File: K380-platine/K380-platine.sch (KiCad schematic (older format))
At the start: 32 parts, among them J1 JST-PH 2, J2 Conn_01x23, J3 MicroMod-M.2E, J4 USB_C_Receptacle_USB2.0, J5 Conn_ARM_JTAG_SWD_10, Q1 PMost Enc FET -20V, Q2 Q_NMOS_DGS, SW1 EG1215AA, SW2 SW_Push, SW3 SW_Push, U1 XC6220B331MR, U2 MCP73831-2-OT

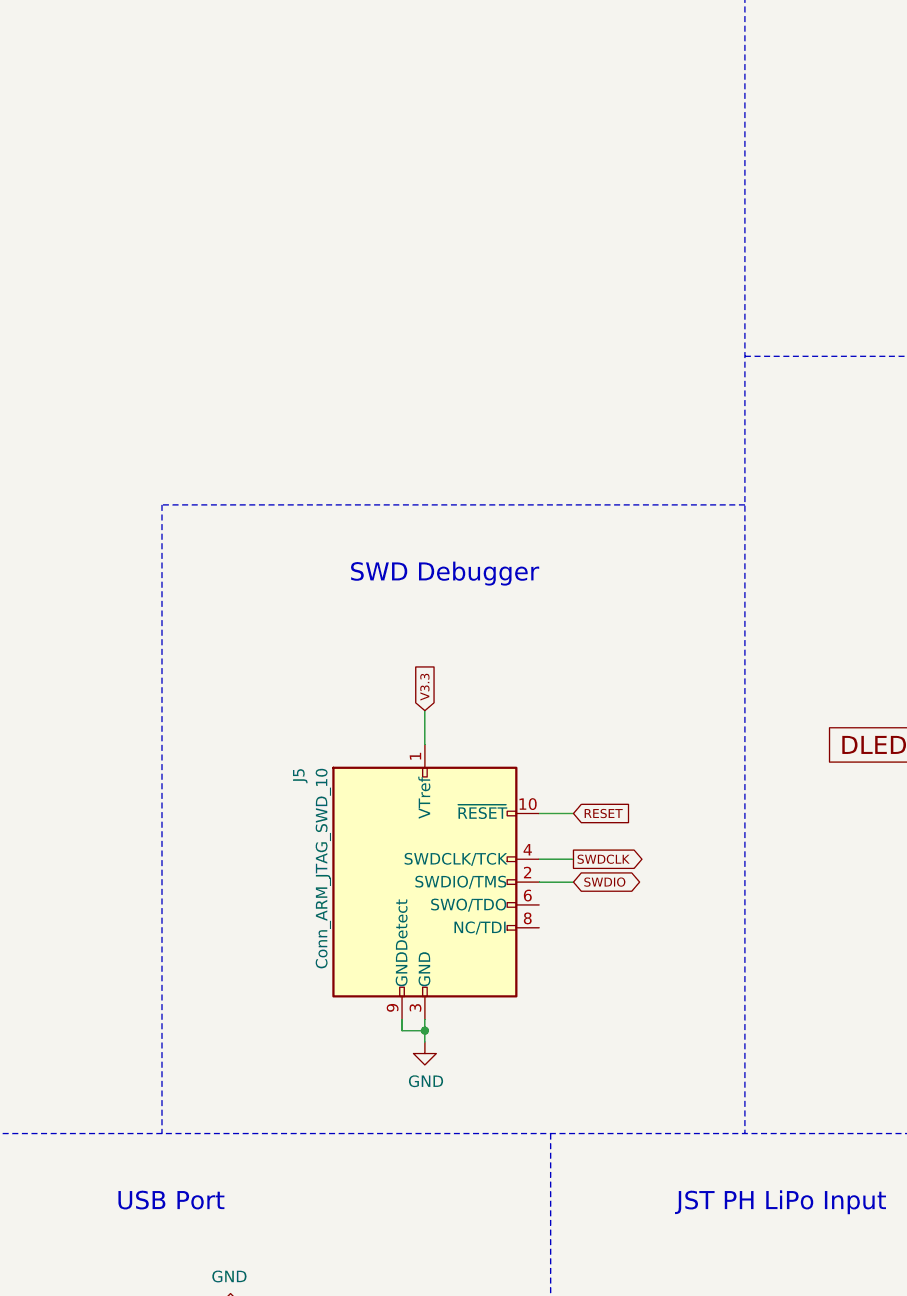
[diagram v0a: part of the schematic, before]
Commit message: Add test probes
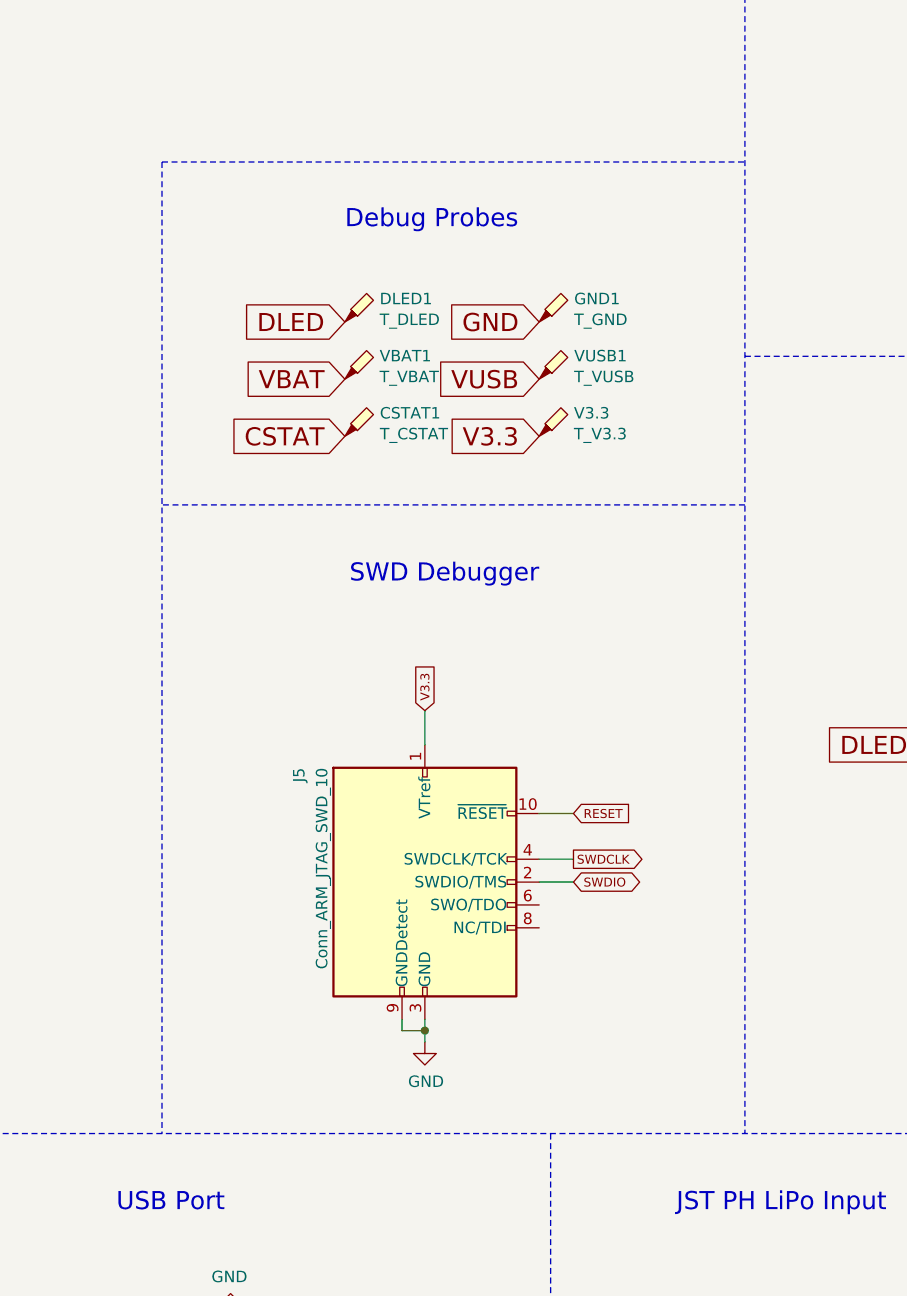
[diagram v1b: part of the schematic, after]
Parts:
- added CSTAT1: T_CSTAT, TestPoint:TestPoint_Pad_D1.0mm, symbol Connector:TestPoint_Probe
- added DLED1: T_DLED, TestPoint:TestPoint_Pad_D1.0mm, symbol Connector:TestPoint_Probe
- added GND1: T_GND, TestPoint:TestPoint_Pad_D1.0mm, symbol Connector:TestPoint_Probe
- added V3.3: T_V3.3, TestPoint:TestPoint_Pad_D1.0mm, symbol Connector:TestPoint_Probe
- added VBAT1: T_VBAT, TestPoint:TestPoint_Pad_D1.0mm, symbol Connector:TestPoint_Probe
- added VUSB1: T_VUSB, TestPoint:TestPoint_Pad_D1.0mm, symbol Connector:TestPoint_Probe
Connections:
- net CSTAT: now also CSTAT1.1
- net DLED: now also DLED1.1
- net GND: now also GND1.1
- net V3.3: now also V3.3.1
- net VBAT: now also VBAT1.1
- net VUSB: now also VUSB1.1
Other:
- note added: "Debug Probes"
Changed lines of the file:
@@
 Wire Notes Line
 	11600 5200 9050 5200
-Wire Notes Line
-	9050 5200 9050 7950
 Text GLabel 4200 3400 0    39   Input ~ 0
 SWDCLK
@@
 Text GLabel 4200 3900 0    39   Output ~ 0
 ROW6
+$Comp
+L Connector:TestPoint_Probe GND1
+U 1 1 62ED9230
+P 10700 4400
+F 0 "GND1" H 10853 4501 50  0000 L CNN
+F 1 "T_GND" H 10853 4410 50  0000 L CNN
+F 2 "TestPoint:TestPoint_Pad_D1.0mm" H 10900 4400 50  0001 C CNN
+F 3 "~" H 10900 4400 50  0001 C CNN
+	1    10700 4400
+	1    0    0    -1
+$EndComp
+$Comp
+L Connector:TestPoint_Probe VUSB1
+U 1 1 62EDA376
+P 10700 4650
+F 0 "VUSB1" H 10853 4751 50  0000 L CNN
+F 1 "T_VUSB" H 10853 4660 50  0000 L CNN
+F 2 "TestPoint:TestPoint_Pad_D1.0mm" H 10900 4650 50  0001 C CNN
+F 3 "~" H 10900 4650 50  0001 C CNN
+	1    10700 4650
+	1    0    0    -1
+$EndComp
+$Comp
+L Connector:TestPoint_Probe V3.3
+U 1 1 62EDAC40
+P 10700 4900
+F 0 "V3.3" H 10852 5001 50  0000 L CNN
+F 1 "T_V3.3" H 10852 4910 50  0000 L CNN
+F 2 "TestPoint:TestPoint_Pad_D1.0mm" H 10900 4900 50  0001 C CNN
+F 3 "~" H 10900 4900 50  0001 C CNN
+	1    10700 4900
+	1    0    0    -1
+$EndComp
+Text GLabel 10700 4900 0    79   Input ~ 0
+V3.3
+Text GLabel 10700 4650 0    79   Input ~ 0
+VUSB
+Text GLabel 10700 4400 0    79   Input ~ 0
+GND
+$Comp
+L Connector:TestPoint_Probe DLED1
+U 1 1 62F54153
+P 9850 4400
+F 0 "DLED1" H 10002 4501 50  0000 L CNN
+F 1 "T_DLED" H 10002 4410 50  0000 L CNN
+F 2 "TestPoint:TestPoint_Pad_D1.0mm" H 10050 4400 50  0001 C CNN
+F 3 "~" H 10050 4400 50  0001 C CNN
+	1    9850 4400
+	1    0    0    -1
+$EndComp
+Text GLabel 9850 4400 0    79   Input ~ 0
+DLED
+$Comp
+L Connector:TestPoint_Probe VBAT1
+U 1 1 62F5DCAD
+P 9850 4650
+F 0 "VBAT1" H 10002 4751 50  0000 L CNN
+F 1 "T_VBAT" H 10002 4660 50  0000 L CNN
+F 2 "TestPoint:TestPoint_Pad_D1.0mm" H 10050 4650 50  0001 C CNN
+F 3 "~" H 10050 4650 50  0001 C CNN
+	1    9850 4650
+	1    0    0    -1
+$EndComp
+Text GLabel 9850 4650 0    79   Input ~ 0
+VBAT
+Text GLabel 9850 4900 0    79   Input ~ 0
+CSTAT
+$Comp
+L Connector:TestPoint_Probe CSTAT1
+U 1 1 62F5F6A8
+P 9850 4900
+F 0 "CSTAT1" H 10003 5001 50  0000 L CNN
+F 1 "T_CSTAT" H 10003 4910 50  0000 L CNN
+F 2 "TestPoint:TestPoint_Pad_D1.0mm" H 10050 4900 50  0001 C CNN
+F 3 "~" H 10050 4900 50  0001 C CNN
+	1    9850 4900
+	1    0    0    -1
+$EndComp
+Text Notes 9850 4000 0    79   ~ 0
+Debug Probes
+Wire Notes Line
+	9050 3700 11600 3700
+Wire Notes Line
+	9050 3700 9050 7950
 $EndSCHEMATC
